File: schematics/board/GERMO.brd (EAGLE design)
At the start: 72.1 x 32 mm, 35 parts

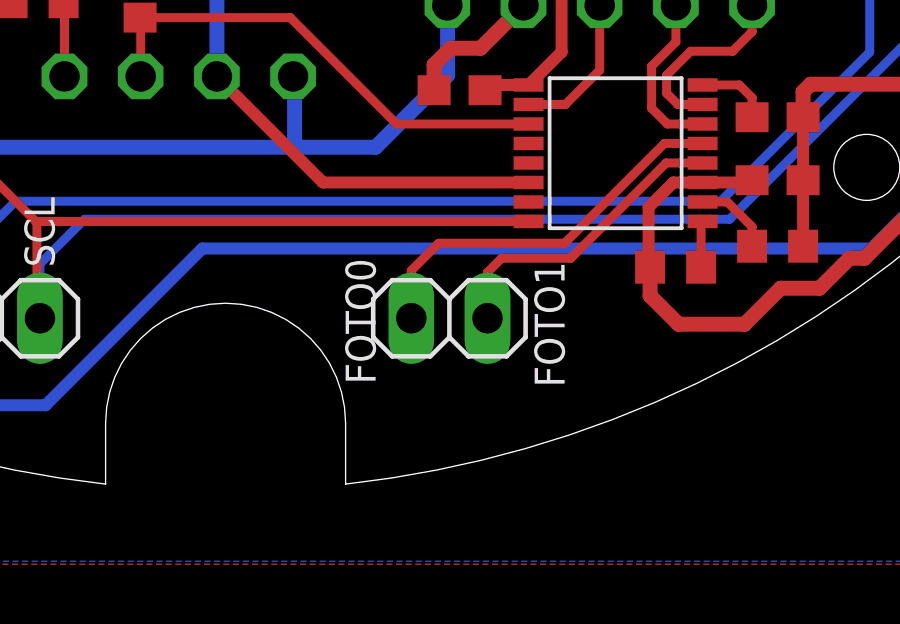
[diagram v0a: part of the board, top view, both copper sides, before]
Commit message: проверка плат
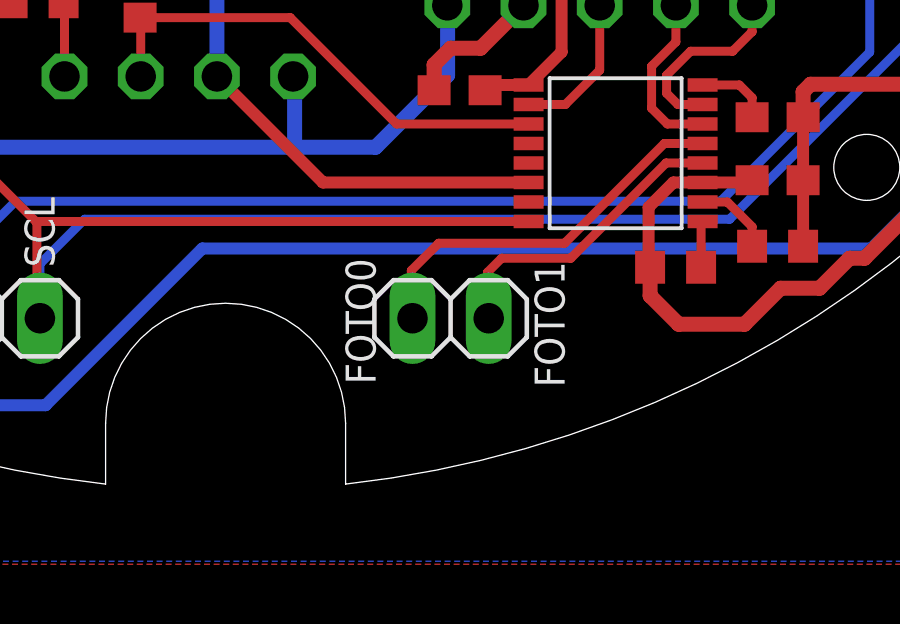
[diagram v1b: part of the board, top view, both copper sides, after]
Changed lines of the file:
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@@
 <?xml version="1.0" encoding="utf-8"?>
 <!DOCTYPE eagle SYSTEM "eagle.dtd">
-<eagle version="9.6.2">
+<eagle version="9.4.2">
 <drawing>
 <settings>
-<setting alwaysvectorfont="no"/>
+<setting alwaysvectorfont="yes"/>
 <setting verticaltext="up"/>
 </settings>
@@
 <attribute name="VALUE" x="56.435" y="9.905" size="1.27" layer="27" font="vector" ratio="15" rot="R180"/>
 </element>
-<element name="JP2" library="pinhead" library_urn="urn:adsk.eagle:library:325" package="1X02" package3d_urn="urn:adsk.eagle:package:22435/2" value="" x="47.46" y="9.5" smashed="yes" rot="R180">
-<attribute name="POPULARITY" value="98" x="47.46" y="9.5" size="1.778" layer="27" rot="R180" display="off"/>
-<attribute name="VALUE" x="50" y="12.675" size="1.27" layer="27" rot="R180"/>
+<element name="JP2" library="pinhead" library_urn="urn:adsk.eagle:library:325" package="1X02" package3d_urn="urn:adsk.eagle:package:22435/2" value="" x="47.5" y="9.5" smashed="yes" rot="R180">
+<attribute name="POPULARITY" value="98" x="47.5" y="9.5" size="1.778" layer="27" rot="R180" display="off"/>
+<attribute name="VALUE" x="50.04" y="12.675" size="1.27" layer="27" rot="R180"/>
 </element>
 </elements>
@@
 <wire x1="55.9" y1="14.675" x2="54.6821125" y2="14.675" width="0.3" layer="1"/>
 <wire x1="54.6821125" y1="14.675" x2="51.5071125" y2="11.5" width="0.3" layer="1"/>
-<wire x1="48.73" y1="11.03" x2="48.73" y2="9.5" width="0.3" layer="1"/>
+<wire x1="48.73" y1="11.03" x2="48.77" y2="9.5" width="0.3" layer="1"/>
 <wire x1="51.5071125" y1="11.5" x2="49.2" y2="11.5" width="0.3" layer="1"/>
 <wire x1="49.2" y1="11.5" x2="48.73" y2="11.03" width="0.3" layer="1"/>
@@
 <contactref element="JP2" pad="2"/>
 <wire x1="55.9" y1="15.325" x2="54.625" y2="15.325" width="0.3" layer="1"/>
-<wire x1="46.19" y1="11.09" x2="46.19" y2="9.5" width="0.3" layer="1"/>
+<wire x1="46.19" y1="11.09" x2="46.23" y2="9.5" width="0.3" layer="1"/>
 <wire x1="54.625" y1="15.325" x2="51.3" y2="12" width="0.3" layer="1"/>
 <wire x1="51.3" y1="12" x2="47.1" y2="12" width="0.3" layer="1"/>
